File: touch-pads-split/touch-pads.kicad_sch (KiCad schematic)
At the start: 19 parts, among them J1 Conn_01x06_Socket, J2 Conn_01x06_Socket, K1 Conn_01x01, K2 Conn_01x01, K3 Conn_01x01, K4 Conn_01x01, K5 Conn_01x01, K6 Conn_01x01, K7 Conn_01x01, K8 Conn_01x01, U1 CAP1188-1-CP-TR

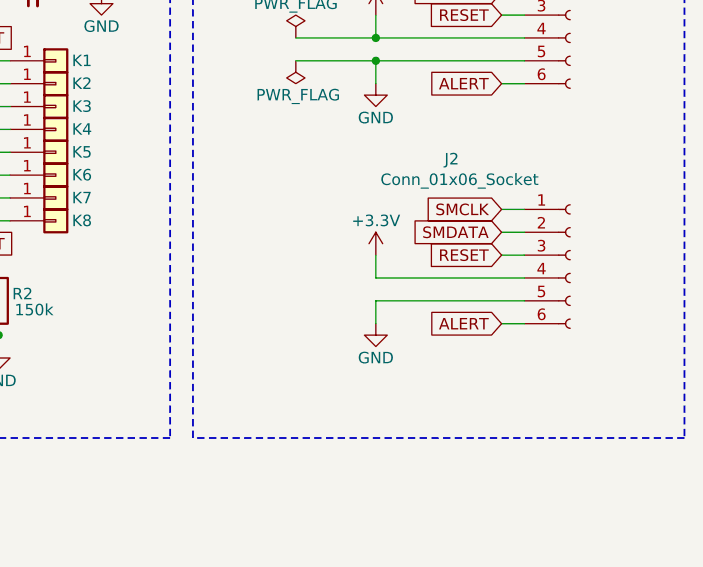
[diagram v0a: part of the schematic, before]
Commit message: angled jst
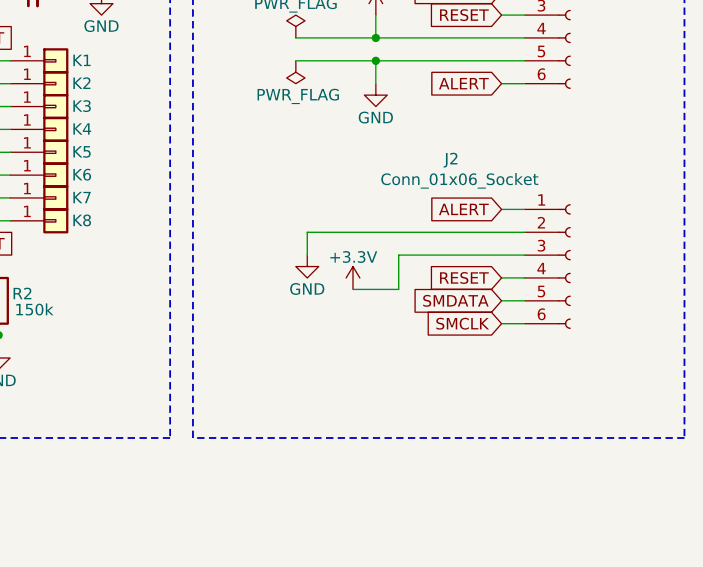
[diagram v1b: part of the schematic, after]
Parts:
- J1, J2: footprint Connector_JST:JST_XH_B6B-XH-A_1x06_P2.50mm_Vertical -> Connector_JST:JST_GH_SM06B-GHS-TB_1x06-1MP_P1.25mm_Horizontal
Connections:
- net +3.3V: now also J2.3 (Pin_3); no longer J2.4 (Pin_4)
- net ALERT: now also J2.1 (Pin_1); no longer J2.6 (Pin_6)
- net GND: now also J2.2 (Pin_2); no longer J2.5 (Pin_5)
- net RESET: now also J2.4 (Pin_4); no longer J2.3 (Pin_3)
- net SMCLK: now also J2.6 (Pin_6); no longer J2.1 (Pin_1)
- net SMDATA: now also J2.5 (Pin_5); no longer J2.2 (Pin_2)

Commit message: add variant resistors
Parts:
- R2: i2c_0x2A (none) -> 120k; i2c_0x2B (none) -> 100k; i2c_0x2C (none) -> 82k
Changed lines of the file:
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@@
+			)
+		)
+		(property "i2c_0x2A" "120k"
+			(at 107.95 66.04 0)
+			(effects
+				(font
+					(size 1.27 1.27)
+				)
+				(hide yes)
+			)
+		)
+		(property "i2c_0x2B" "100k"
+			(at 107.95 66.04 0)
+			(effects
+				(font
+					(size 1.27 1.27)
+				)
+				(hide yes)
+			)
+		)
+		(property "i2c_0x2C" "82k"
+			(at 107.95 66.04 0)
+			(effects
+				(font
+					(size 1.27 1.27)
+				)
+				(hide yes)
 			)
 		)
